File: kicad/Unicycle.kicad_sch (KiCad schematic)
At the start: 18 parts, among them IC1 TSR 2 2450, P3 Battery Connector, P4 Safety Switch Connector, P5 Motor Driver Connector, P6 IMU Connector, U1 Teensy4.0

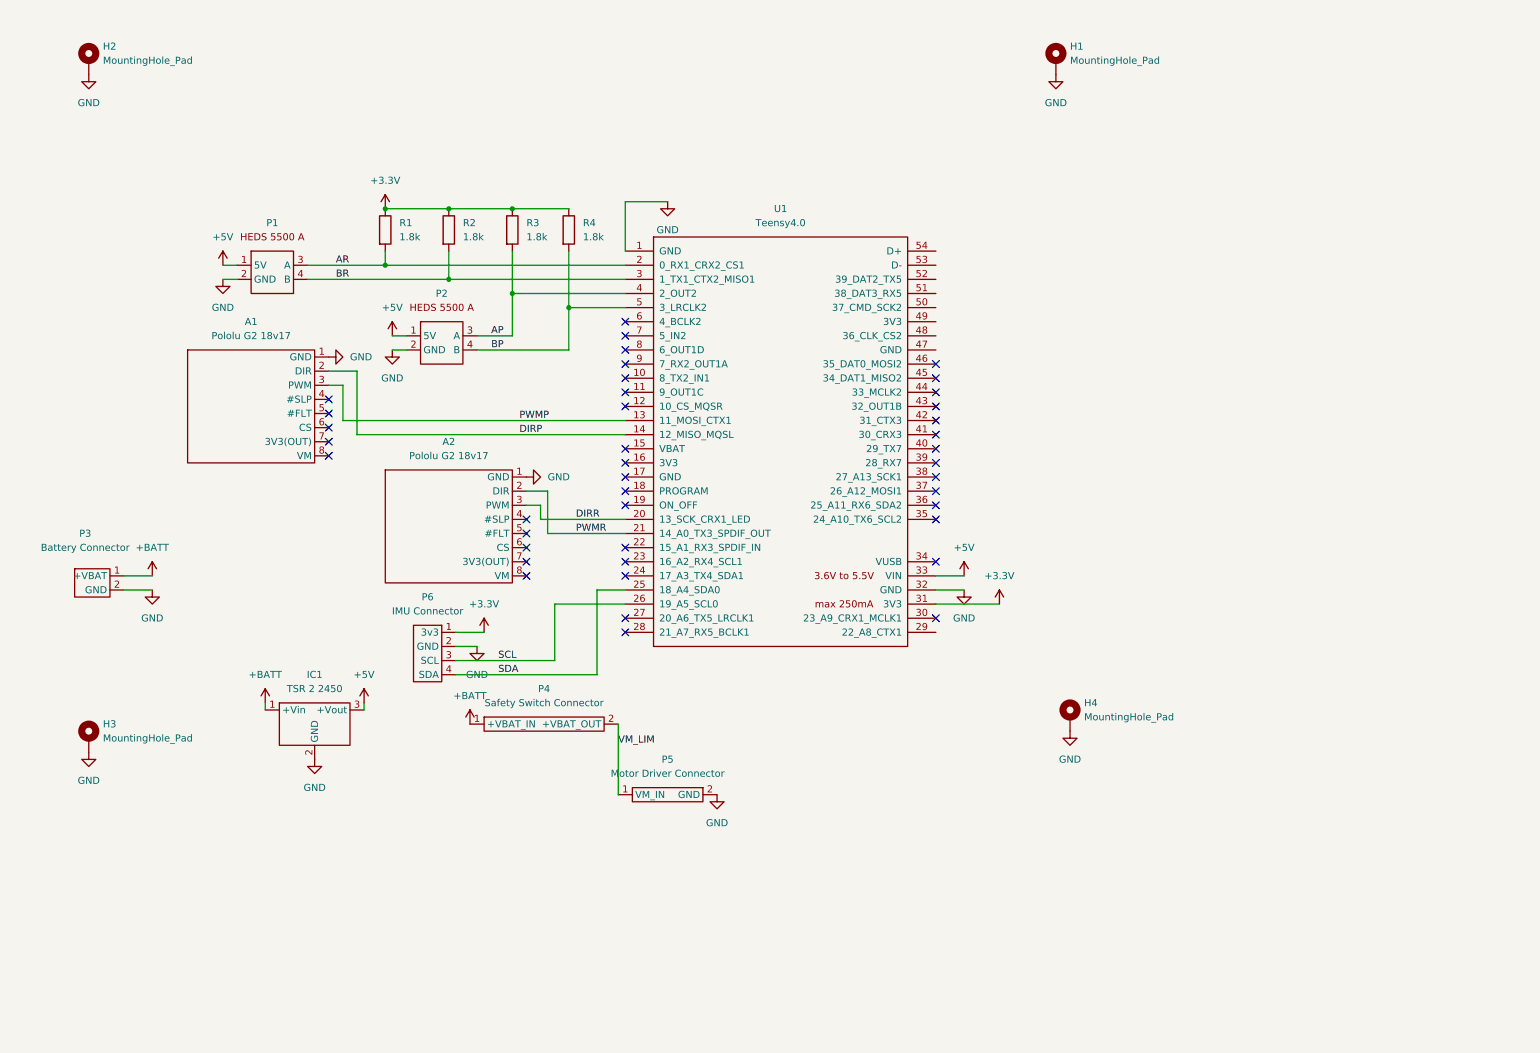
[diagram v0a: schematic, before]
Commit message: update
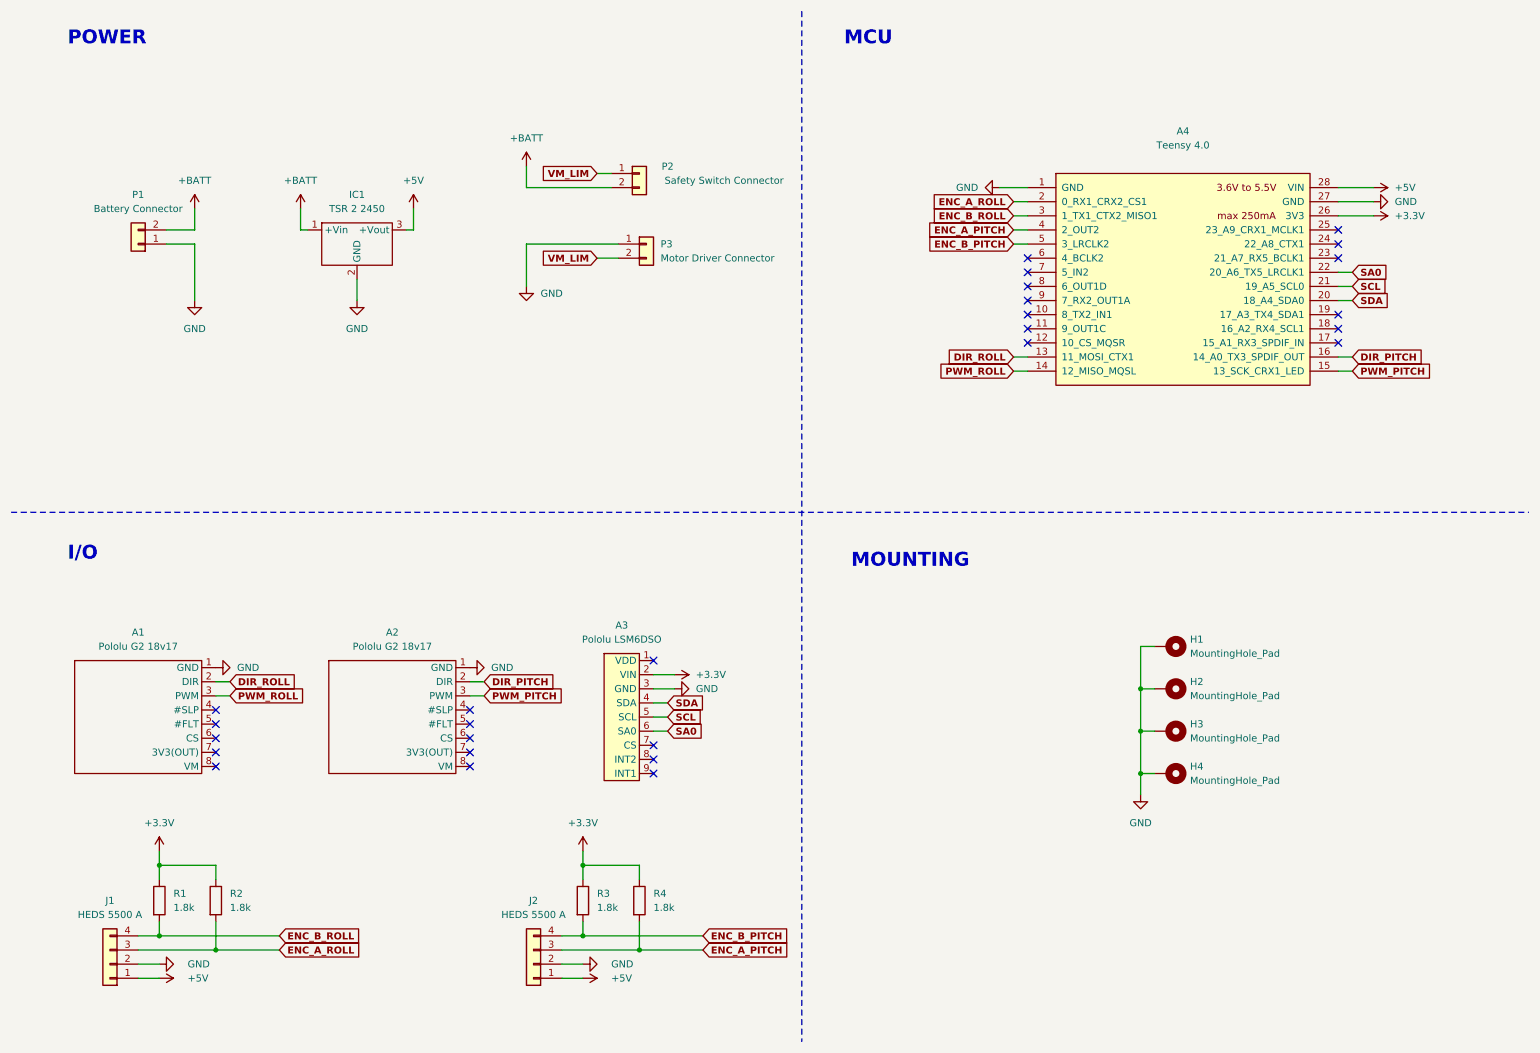
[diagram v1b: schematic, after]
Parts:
- removed P1, P2: ~, Connector_PinHeader_2.54mm:PinHeader_1x04_P2.54mm_Vertical, symbol unicycle:Quad_Connector
- removed P6: IMU Connector, Connector_PinHeader_2.54mm:PinHeader_1x04_P2.54mm_Vertical, symbol unicycle_lib:IMU Connector
- removed U1: Teensy4.0, teensy_foot:Teensy40, symbol teensy_lib:Teensy4.0
- added A3: Pololu LSM6DSO, unicycle_foot:PololuLSM6DSO Text Up, symbol unicycle_lib:Pololu LSM6DSO
- added A4: Teensy 4.0, unicycle_foot:Teensy40 Simple, symbol unicycle_lib:Teensy4.0 Simple
- added J1, J2: HEDS 5500 A, Connector_PinHeader_2.54mm:PinHeader_1x04_P2.54mm_Vertical, symbol Connector_Generic:Conn_01x04
- A1, A2: footprint unicycle_foot:Pololu G2 18v17 -> unicycle_foot:Pololu G2 18v17 Text Up
- P1: renamed from P3; footprint Connector_PinHeader_2.54mm:PinHeader_1x02_P2.54mm_Vertical -> Connector_AMASS:AMASS_XT60-F_1x02_P7.20mm_Vertical; symbol unicycle_lib:Battery Connector -> Connector_Generic:Conn_01x02
- P2: renamed from P4; footprint Connector_PinHeader_2.54mm:PinHeader_1x02_P2.54mm_Vertical -> Connector_AMASS:AMASS_XT60-F_1x02_P7.20mm_Vertical; symbol unicycle_lib:Safety Switch Connector -> Connector_Generic:Conn_01x02
- P3: renamed from P5; footprint Connector_PinHeader_2.54mm:PinHeader_1x02_P2.54mm_Vertical -> Connector_AMASS:AMASS_XT60-F_1x02_P7.20mm_Vertical; symbol unicycle_lib:Motor Driver Connector -> Connector_Generic:Conn_01x02
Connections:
- net +3.3V: now also A3.2 (VIN), A4.26 (3V3)
- net +5V: now also A4.28 (VIN), J1.1 (Pin_1), J2.1 (Pin_1)
- net +BATT: now also P1.2 (Pin_2), P2.2 (Pin_2); no longer P1.1 (+VBAT), P2.1 (+VBAT_IN)
- net GND: now also P1.1 (Pin_1), P3.1 (Pin_1), A3.3 (GND), A4.1 (GND), A4.27 (GND), J1.2 (Pin_2), J2.2 (Pin_2); no longer P1.2 (GND), P3.2 (GND)
- net SCL: now also A3.5 (SCL), A4.21 (19_A5_SCL0)
- net SDA: now also A3.4 (SDA), A4.20 (18_A4_SDA0)
- net VM_LIM: now also P2.1 (Pin_1), P3.2 (Pin_2); no longer P2.2 (+VBAT_OUT), P3.1 (VM_IN)
- net AP renamed ENC_B_PITCH
- net ENC_B_PITCH: now also A4.5 (3_LRCLK2), J2.4 (Pin_4)
- net AR renamed ENC_B_ROLL
- net ENC_B_ROLL: now also A4.3 (1_TX1_CTX2_MISO1), J1.4 (Pin_4)
- net BP renamed ENC_A_PITCH
- net ENC_A_PITCH: now also A4.4 (2_OUT2), J2.3 (Pin_3)
- net BR renamed ENC_A_ROLL
- net ENC_A_ROLL: now also A4.2 (0_RX1_CRX2_CS1), J1.3 (Pin_3)
- net DIRP renamed DIR_ROLL
- net DIR_ROLL: now also A4.13 (11_MOSI_CTX1)
- net DIRR renamed PWM_PITCH
- net PWM_PITCH: now also A4.15 (13_SCK_CRX1_LED)
- net PWMP renamed PWM_ROLL
- net PWM_ROLL: now also A4.14 (12_MISO_MQSL)
- net PWMR renamed DIR_PITCH
- net DIR_PITCH: now also A4.16 (14_A0_TX3_SPDIF_OUT)
- new net SA0: A3.6 (SA0), A4.22 (20_A6_TX5_LRCLK1)
- no-connect marks 41 -> 27
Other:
- note added: "I/O"
- note added: "MCU"
- note added: "MOUNTING"
- note added: "POWER"
- moved on the sheet: A1, A2, H1, H2, H3, H4, IC1, R1, R2, R3, R4
